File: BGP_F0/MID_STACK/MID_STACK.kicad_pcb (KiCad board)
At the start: 2 copper layers, 19.5 x 21.5 mm, 7 parts, among them J1 Conn_01x04_Male, P1 CONN_01X09

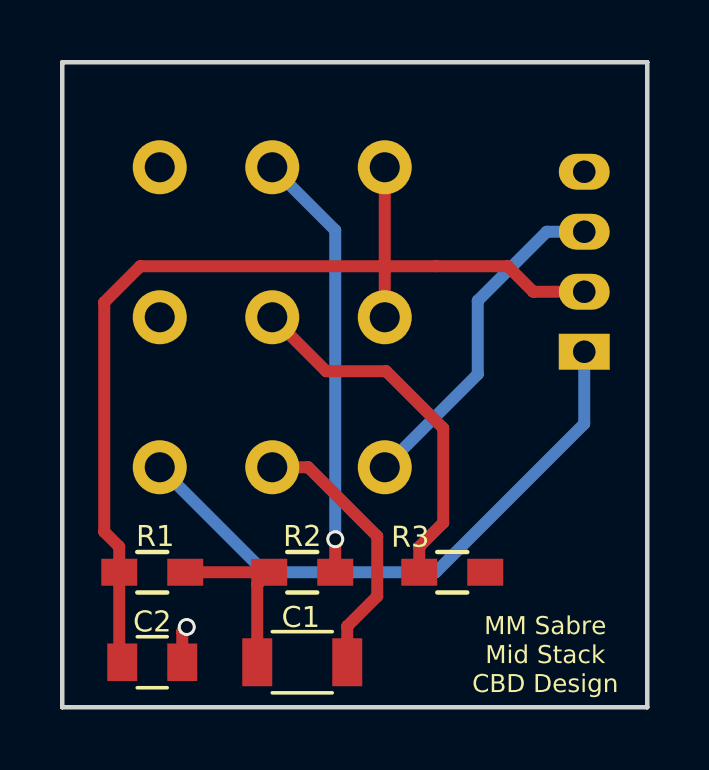
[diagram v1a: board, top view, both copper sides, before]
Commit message: Minor tweaks for MM/F0 - gerbers ready to go out
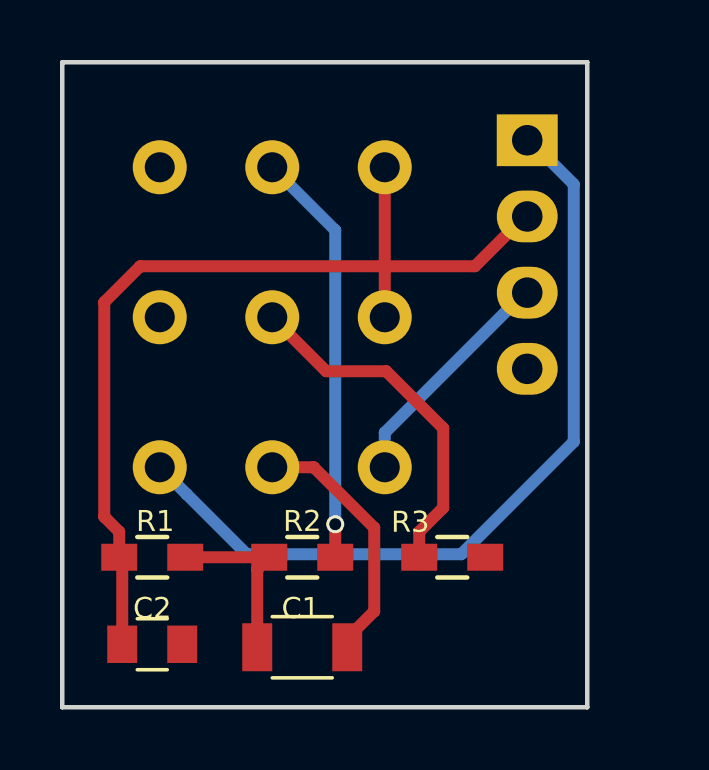
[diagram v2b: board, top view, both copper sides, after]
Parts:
- J1: footprint Connectors_JST:JST_PH_B4B-PH-K_04x2.00mm_Straight -> Pin_Headers:Pin_Header_Straight_1x04
- moved J1 7.30 mm to (144.5, 83.6), turned to 180 degrees
- moved C2 0.60 mm to (132.0, 100.4)
- moved C1 0.50 mm to (137.0, 100.5)
- moved R1 0.50 mm to (132.0, 97.5)
- moved R2 0.50 mm to (137.0, 97.5)
- moved R3 0.50 mm to (142.0, 97.5)
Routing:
- net /MID_I: track 20.1 -> 27.3 mm
- net /MID_O: track 11.3 -> 7.81 mm
- net /MID_R: track 34.2 -> 32.0 mm
- net /Vref: track 1.24 -> 0.00 mm, vias 1 -> 0
- net /F2_2: track 12.4 -> 11.9 mm
- net /F1_2: track 14.4 -> 13.9 mm
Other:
- board size 19.5 x 21.5 mm -> 17.5 x 21.5 mm
- board text removed: "MM Sabre Mid Stack CBD Design"
